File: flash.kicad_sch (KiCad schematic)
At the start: 13 parts, among them U1 ECP5U_12_CABGA256, U11 W25Q128JVS

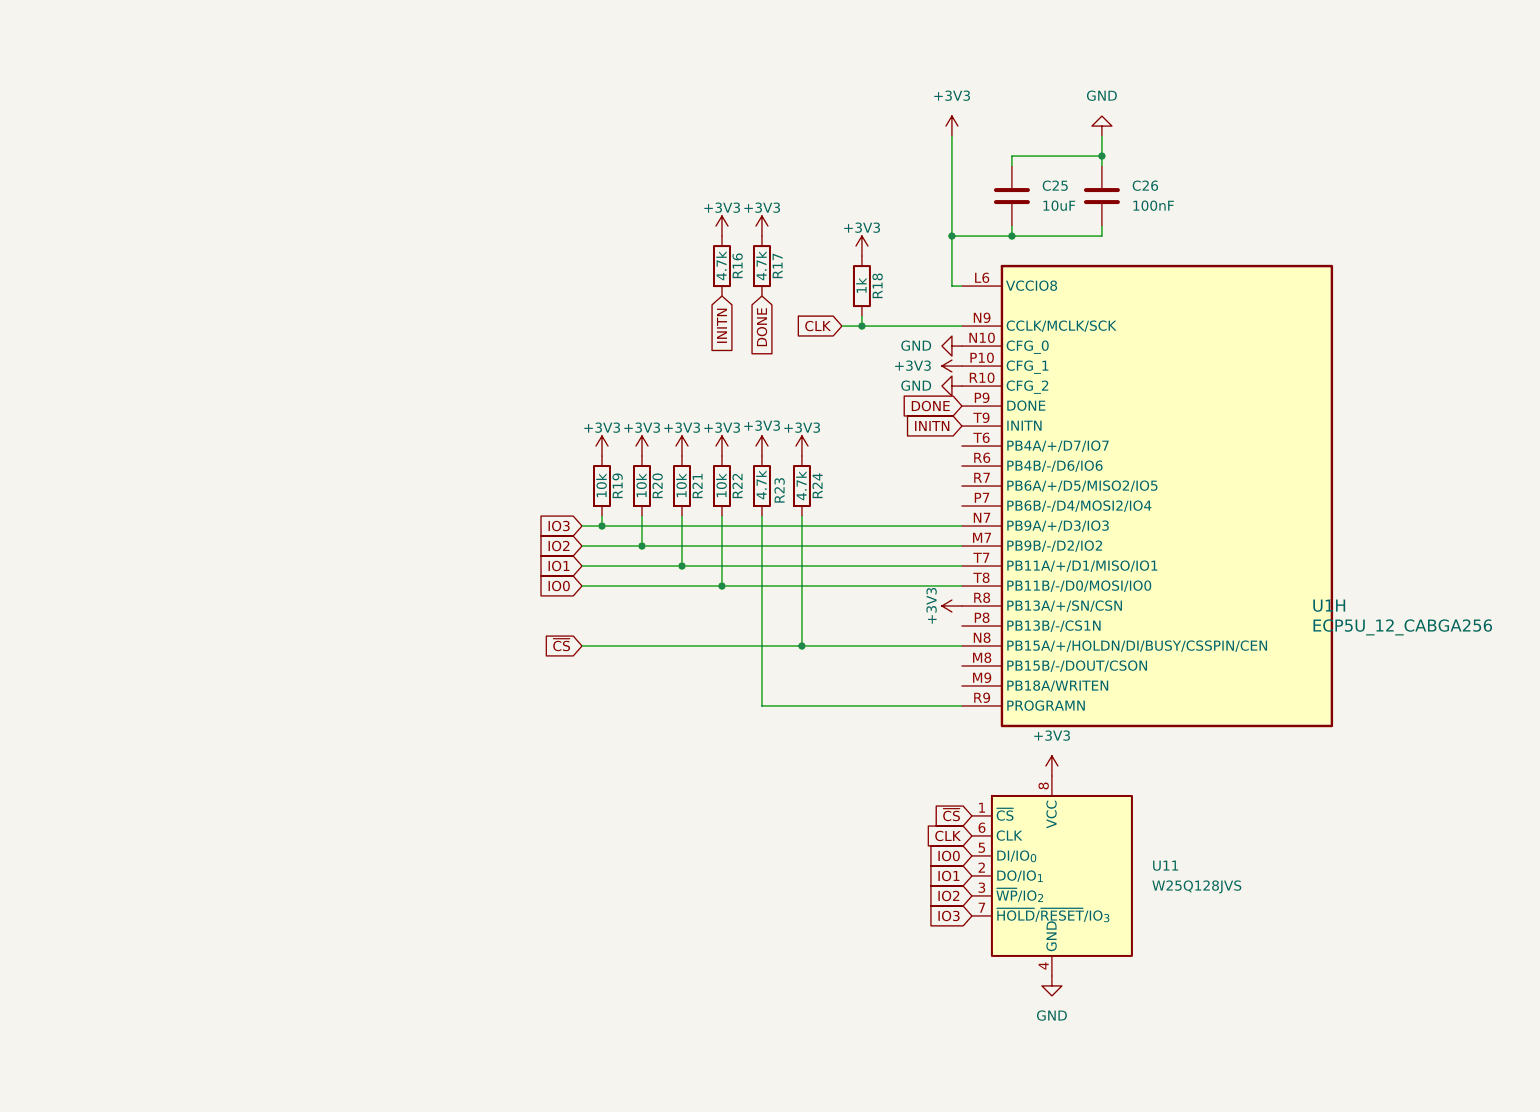
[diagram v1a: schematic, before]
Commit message: Stash
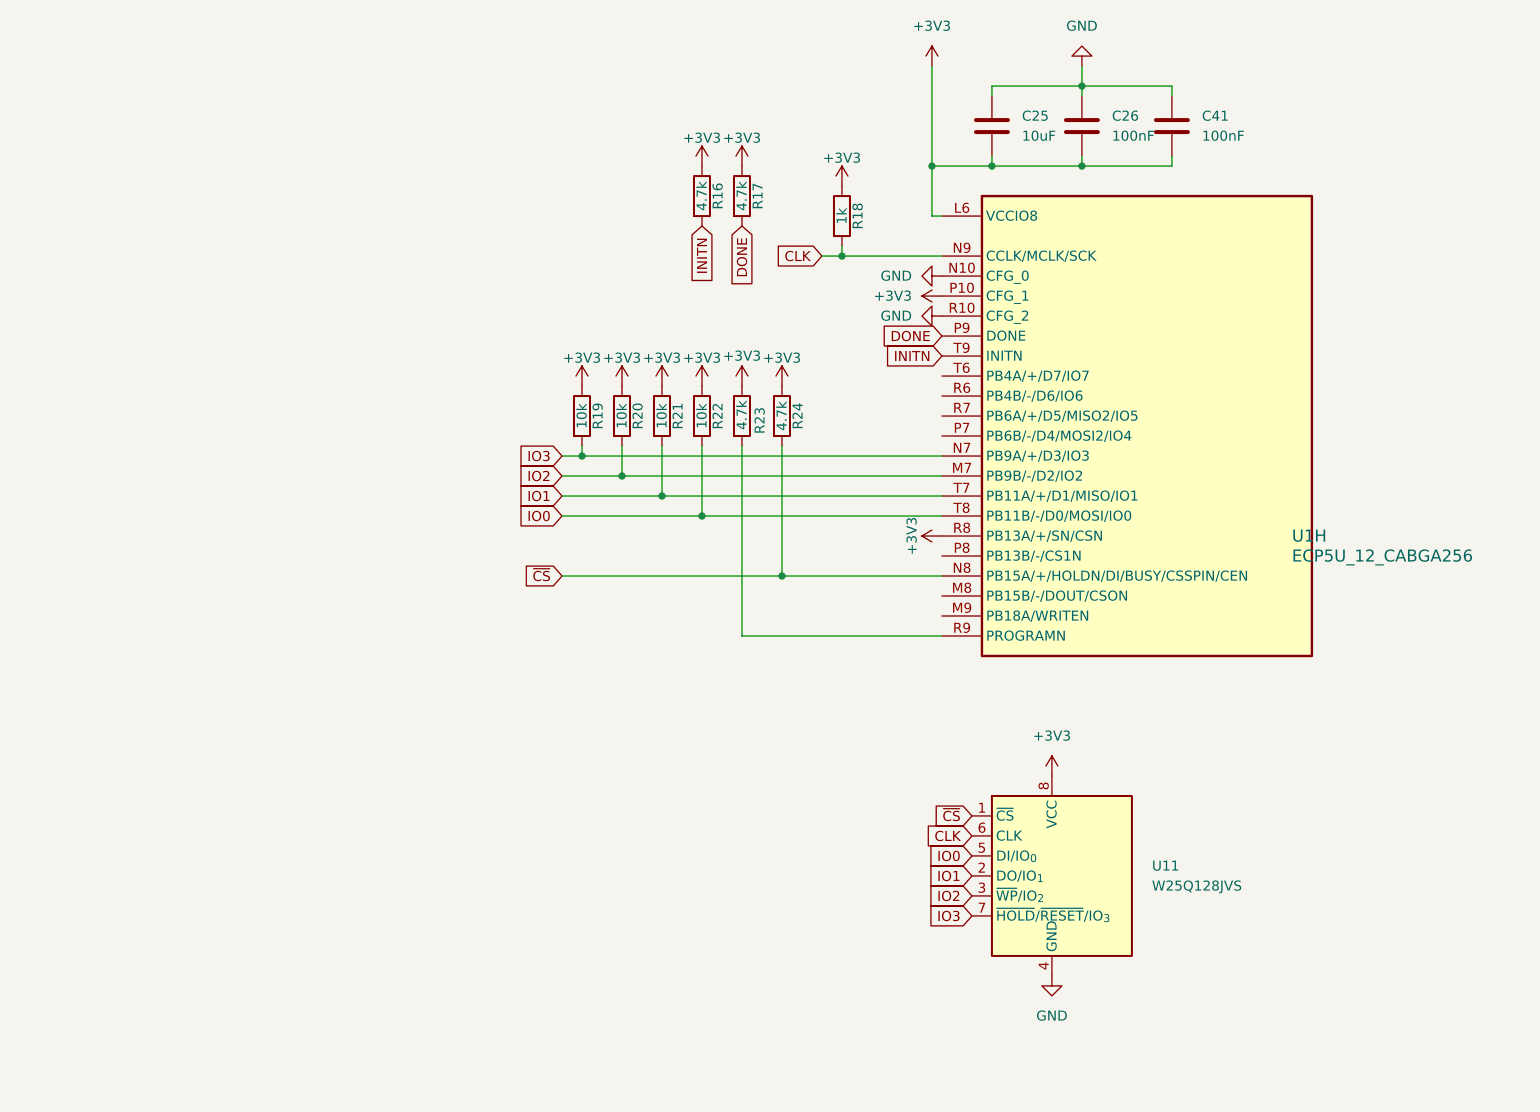
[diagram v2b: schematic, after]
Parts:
- added C41: 100nF, Capacitor_SMD:C_0402_1005Metric, symbol Device:C
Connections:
- net +3V3: now also C41.2
- net GND: now also C41.1
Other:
- moved on the sheet: C25, C26, R16, R17, R18, R19, R20, R21, R22, R23, R24, U1H

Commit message: Rev 1
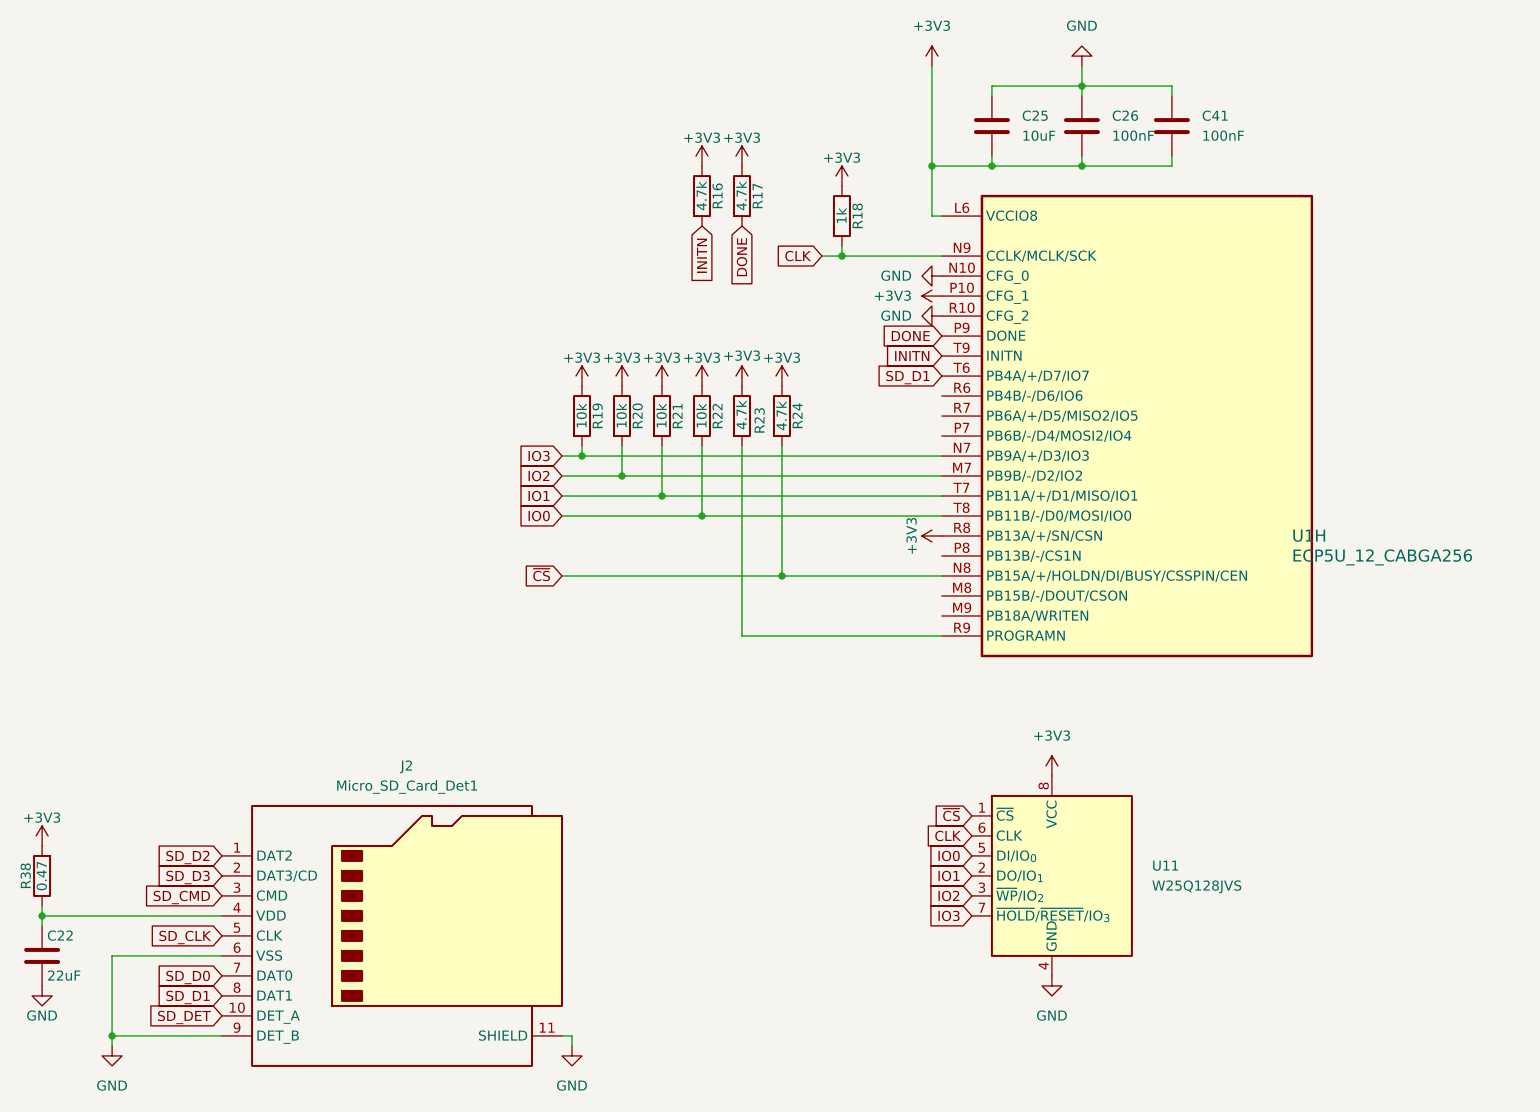
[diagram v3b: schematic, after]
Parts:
- added C22: 22uF, Capacitor_SMD:C_0603_1608Metric, symbol Device:C
- added J2: Micro_SD_Card_Det1, anice-lib:SDCard molex, symbol Connector:Micro_SD_Card_Det2
- added R38: 0.47, Resistor_SMD:R_0603_1608Metric, symbol Device:R
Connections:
- net +3V3: now also R38.2
- net GND: now also C22.2, J2.11 (SHIELD), J2.6 (VSS), J2.9 (DET_B)
- net SD_D1: now reaches U1.T6 (PB4A/+/D7/IO7)
- net SD_D1: now also J2.8 (DAT1)
- new net: C22.1, J2.4 (VDD), R38.1
- new net SD_CLK: J2.5 (CLK)
- new net SD_CMD: J2.3 (CMD)
- new net SD_D0: J2.7 (DAT0)
- new net SD_D2: J2.1 (DAT2)
- new net SD_D3: J2.2 (DAT3/CD)
- new net SD_DET: J2.10 (DET_A)

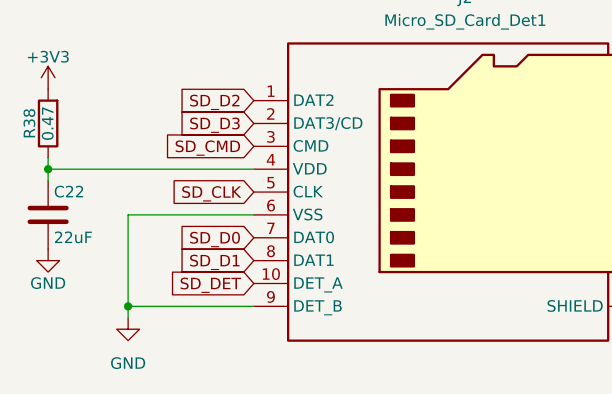
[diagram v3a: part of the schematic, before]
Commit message: No DRC Errors
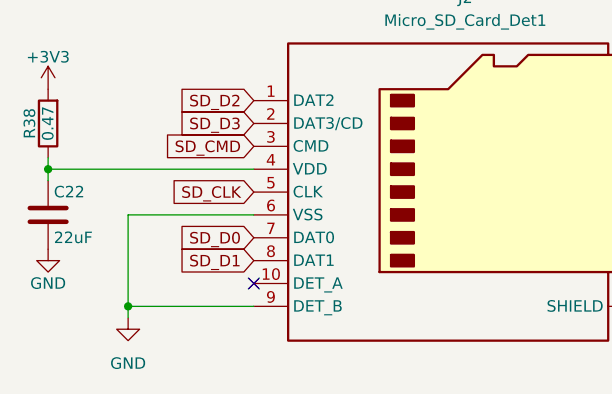
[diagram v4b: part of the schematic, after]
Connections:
- net SD_DET: no longer names the net of J2.10 (DET_A)
- no-connect marks 0 -> 1
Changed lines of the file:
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@@
 		(color 0 0 0 0)
 	)
+	(no_connect
+		(at 58.42 158.75)
+	)
 	(wire
 		(pts
@@
 				(hide yes)
 			)
-		)
-	)
-	(global_label "SD_DET"
-		(shape input)
-		(at 58.42 158.75 180)
-		(effects
-			(font
-				(size 1.27 1.27)
-			)
-			(justify right)
-		)
-		(property "Intersheetrefs" "${INTERSHEET_REFS}"
-			(at 58.42 158.75 0)
-			(effects
-				(font
-					(size 1.27 1.27)
-				)
-				(hide yes)
-			)
